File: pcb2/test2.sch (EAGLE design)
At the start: 56 parts, among them IC1 LMV358M, IC2 LMV358M, IC3 STM32F10XCXT6, Q1 8mhz

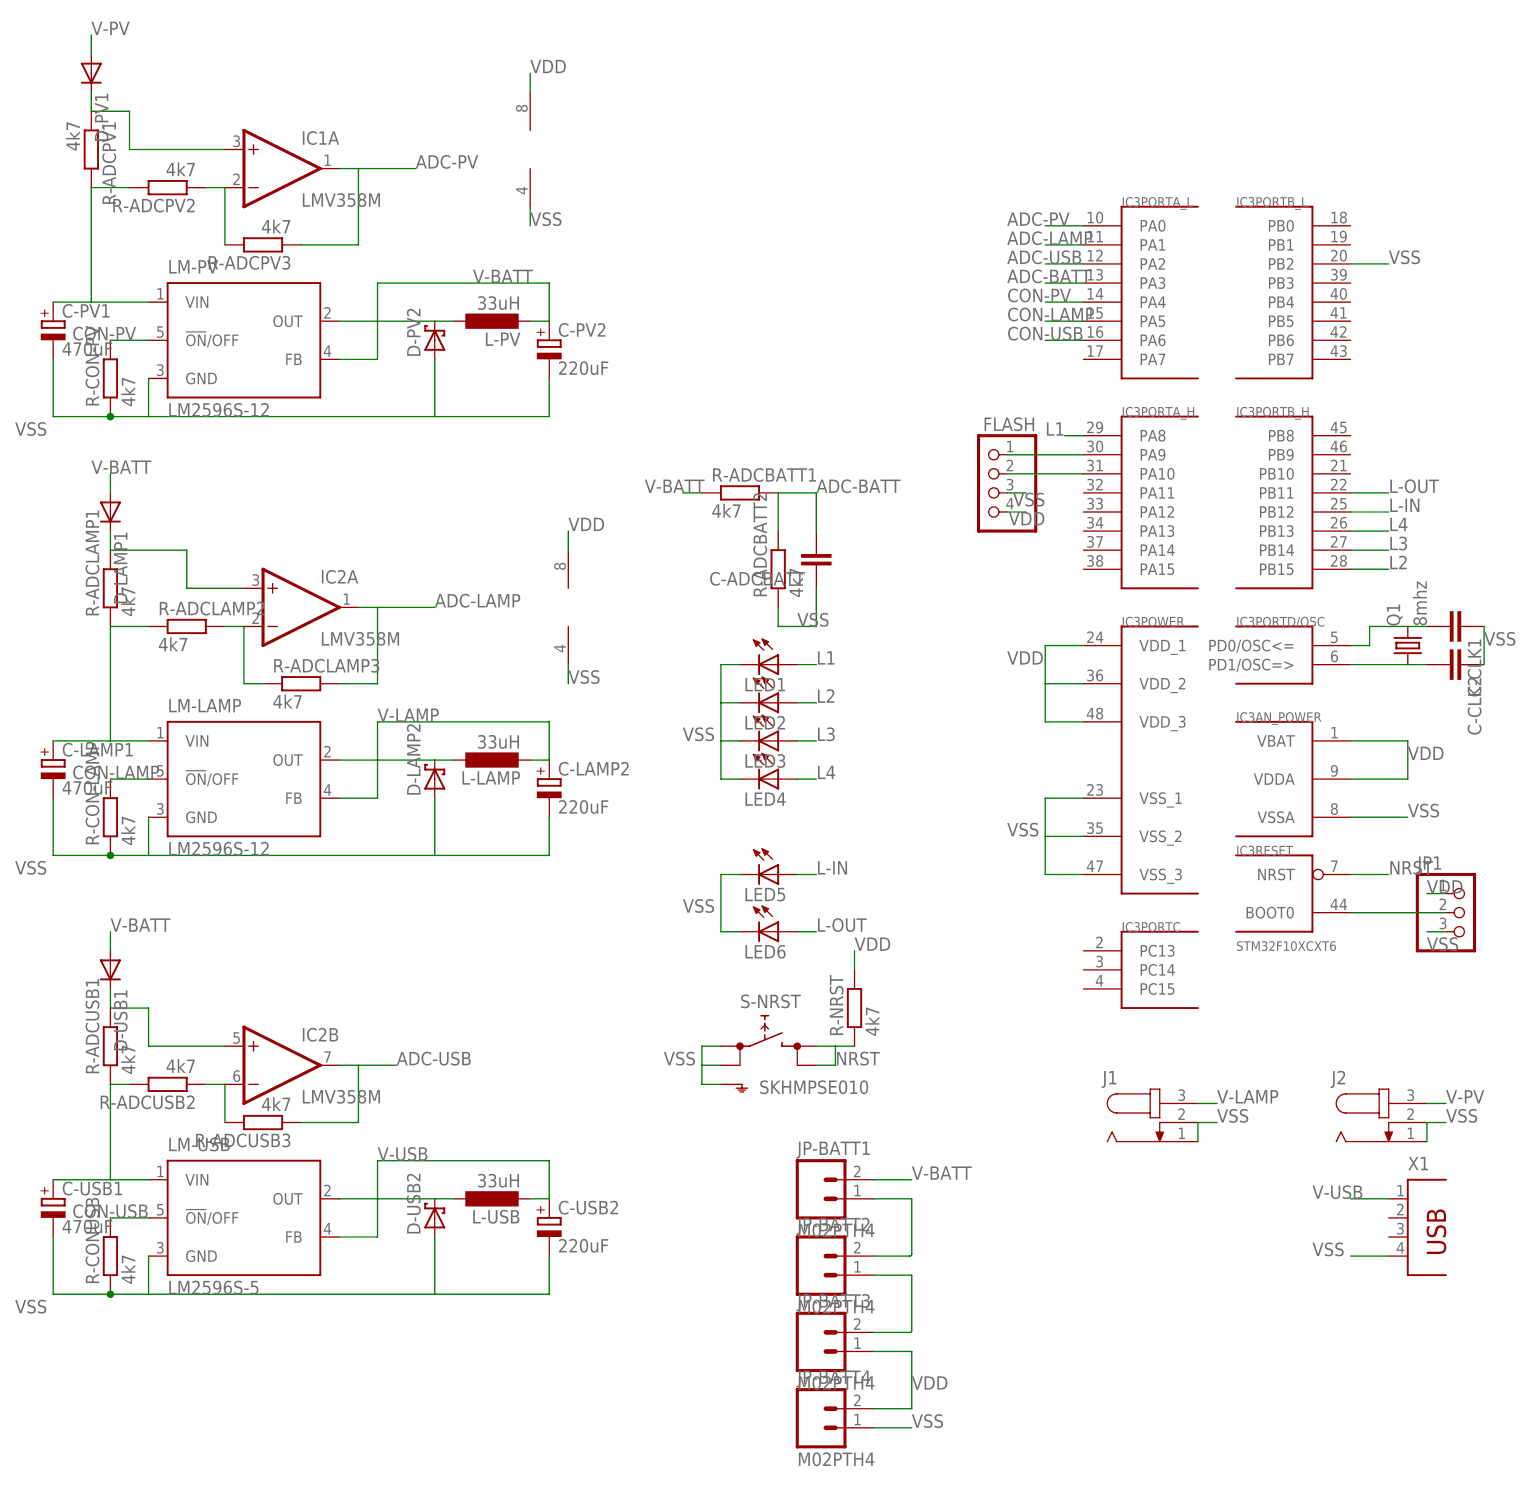
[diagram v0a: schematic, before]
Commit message: ready to facturing
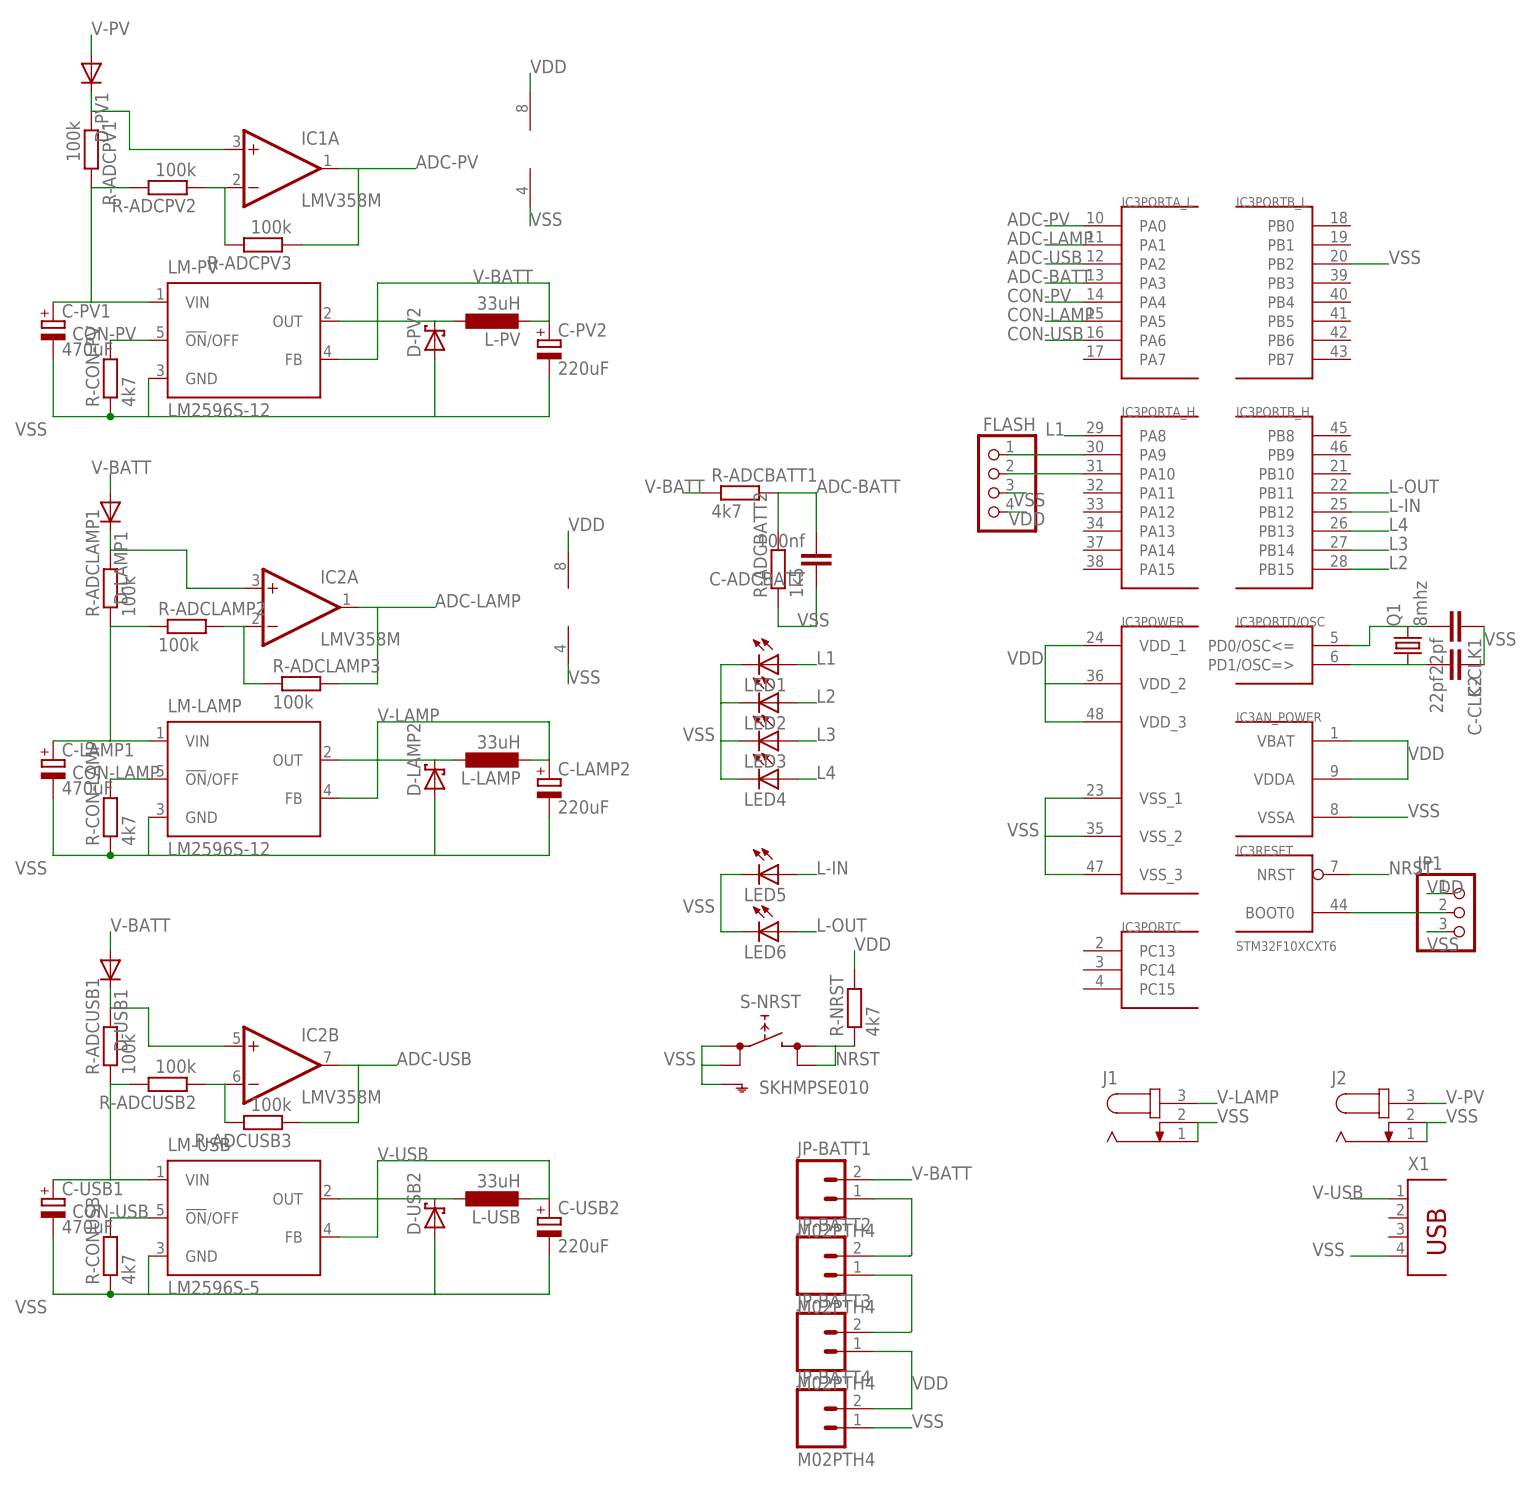
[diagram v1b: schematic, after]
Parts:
- C-ADCBATT: value (none) -> 100nf
- C-CLK1, C-CLK2: value (none) -> 22pf
- R-ADCBATT2: value 4k7 -> 1k5
- R-ADCLAMP1, R-ADCLAMP2, R-ADCLAMP3, R-ADCPV1, R-ADCPV2, R-ADCPV3, R-ADCUSB1, R-ADCUSB2, R-ADCUSB3: value 4k7 -> 100k
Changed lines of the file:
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@@
 <part name="C-USB2" library="resistor" deviceset="CPOL-EU" device="E2.5-5" value="220uF"/>
 <part name="IC1" library="linear" deviceset="LMV358?*" device="M"/>
-<part name="R-ADCPV2" library="resistor" deviceset="R-EU_" device="R0805" value="4k7"/>
-<part name="R-ADCPV1" library="resistor" deviceset="R-EU_" device="R0805" value="4k7"/>
-<part name="R-ADCPV3" library="resistor" deviceset="R-EU_" device="R0805" value="4k7"/>
+<part name="R-ADCPV2" library="resistor" deviceset="R-EU_" device="R0805" value="100k"/>
+<part name="R-ADCPV1" library="resistor" deviceset="R-EU_" device="R0805" value="100k"/>
+<part name="R-ADCPV3" library="resistor" deviceset="R-EU_" device="R0805" value="100k"/>
 <part name="D-PV1" library="diode" deviceset="DIODE-" device="DO-214AC"/>
 <part name="IC2" library="linear" deviceset="LMV358?*" device="M"/>
-<part name="R-ADCLAMP2" library="resistor" deviceset="R-EU_" device="R0805" value="4k7"/>
-<part name="R-ADCLAMP1" library="resistor" deviceset="R-EU_" device="R0805" value="4k7"/>
-<part name="R-ADCLAMP3" library="resistor" deviceset="R-EU_" device="R0805" value="4k7"/>
+<part name="R-ADCLAMP2" library="resistor" deviceset="R-EU_" device="R0805" value="100k"/>
+<part name="R-ADCLAMP1" library="resistor" deviceset="R-EU_" device="R0805" value="100k"/>
+<part name="R-ADCLAMP3" library="resistor" deviceset="R-EU_" device="R0805" value="100k"/>
 <part name="D-LAMP1" library="diode" deviceset="DIODE-" device="DO-214AC"/>
-<part name="R-ADCUSB1" library="resistor" deviceset="R-EU_" device="R0805" value="4k7"/>
-<part name="R-ADCUSB2" library="resistor" deviceset="R-EU_" device="R0805" value="4k7"/>
-<part name="R-ADCUSB3" library="resistor" deviceset="R-EU_" device="R0805" value="4k7"/>
+<part name="R-ADCUSB1" library="resistor" deviceset="R-EU_" device="R0805" value="100k"/>
+<part name="R-ADCUSB2" library="resistor" deviceset="R-EU_" device="R0805" value="100k"/>
+<part name="R-ADCUSB3" library="resistor" deviceset="R-EU_" device="R0805" value="100k"/>
 <part name="D-USB1" library="diode" deviceset="DIODE-" device="DO-214AC"/>
 <part name="LED1" library="led" deviceset="LED" device="CHIP-LED0805"/>
@@
 <part name="LED6" library="led" deviceset="LED" device="CHIP-LED0805"/>
 <part name="R-ADCBATT1" library="resistor" deviceset="R-EU_" device="R0805" value="4k7"/>
-<part name="R-ADCBATT2" library="resistor" deviceset="R-EU_" device="R0805" value="4k7"/>
-<part name="C-ADCBATT" library="resistor" deviceset="C-EU" device="C0805"/>
+<part name="R-ADCBATT2" library="resistor" deviceset="R-EU_" device="R0805" value="1k5"/>
+<part name="C-ADCBATT" library="resistor" deviceset="C-EU" device="C0805" value="100nf"/>
 <part name="S-NRST" library="switch" deviceset="SKHMP*E010" device="" technology="S"/>
 <part name="R-NRST" library="resistor" deviceset="R-EU_" device="R0805" value="4k7"/>
@@
 <part name="JP1" library="pinhead" deviceset="PINHD-1X3" device=""/>
 <part name="Q1" library="crystal" deviceset="CRYSTAL" device="HC49S" value="8mhz"/>
-<part name="C-CLK1" library="resistor" deviceset="C-EU" device="C0805"/>
-<part name="C-CLK2" library="resistor" deviceset="C-EU" device="C0805"/>
+<part name="C-CLK1" library="resistor" deviceset="C-EU" device="C0805" value="22pf"/>
+<part name="C-CLK2" library="resistor" deviceset="C-EU" device="C0805" value="22pf"/>
 <part name="FLASH" library="pinhead" deviceset="PINHD-1X4" device=""/>
 <part name="X1" library="con-berg" deviceset="PN87520" device=""/>
